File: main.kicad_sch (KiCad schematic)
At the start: 19 parts, among them SW1 Switch, SW2 Switch, SW3 Switch, SW4 Switch, SW5 Switch, SW6 Switch, SW7 Switch, SW8 Switch, SW9 Switch

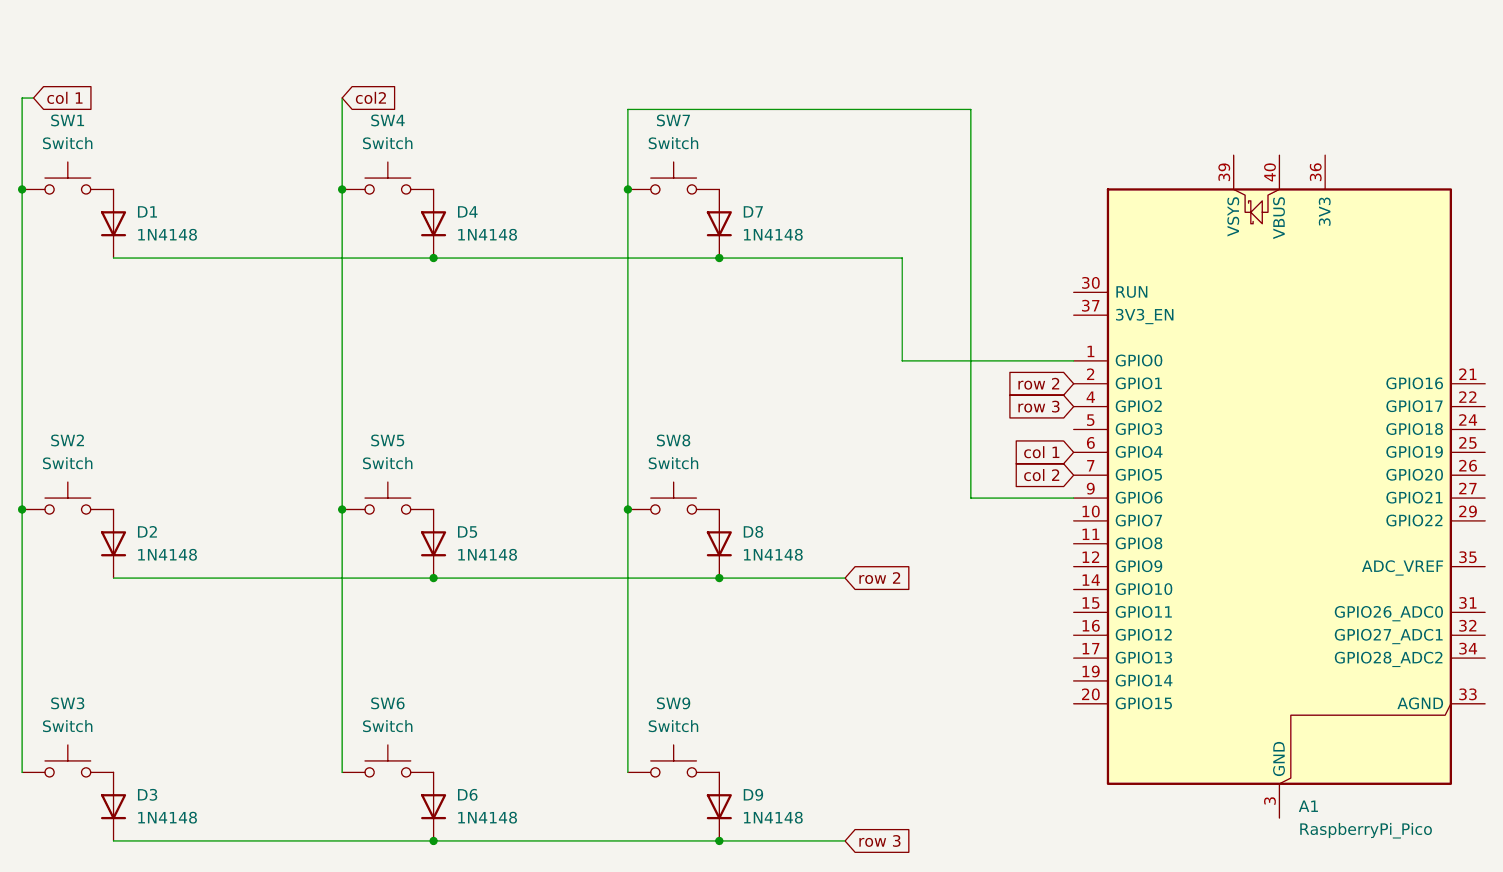
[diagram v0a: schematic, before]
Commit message: fixed pcb
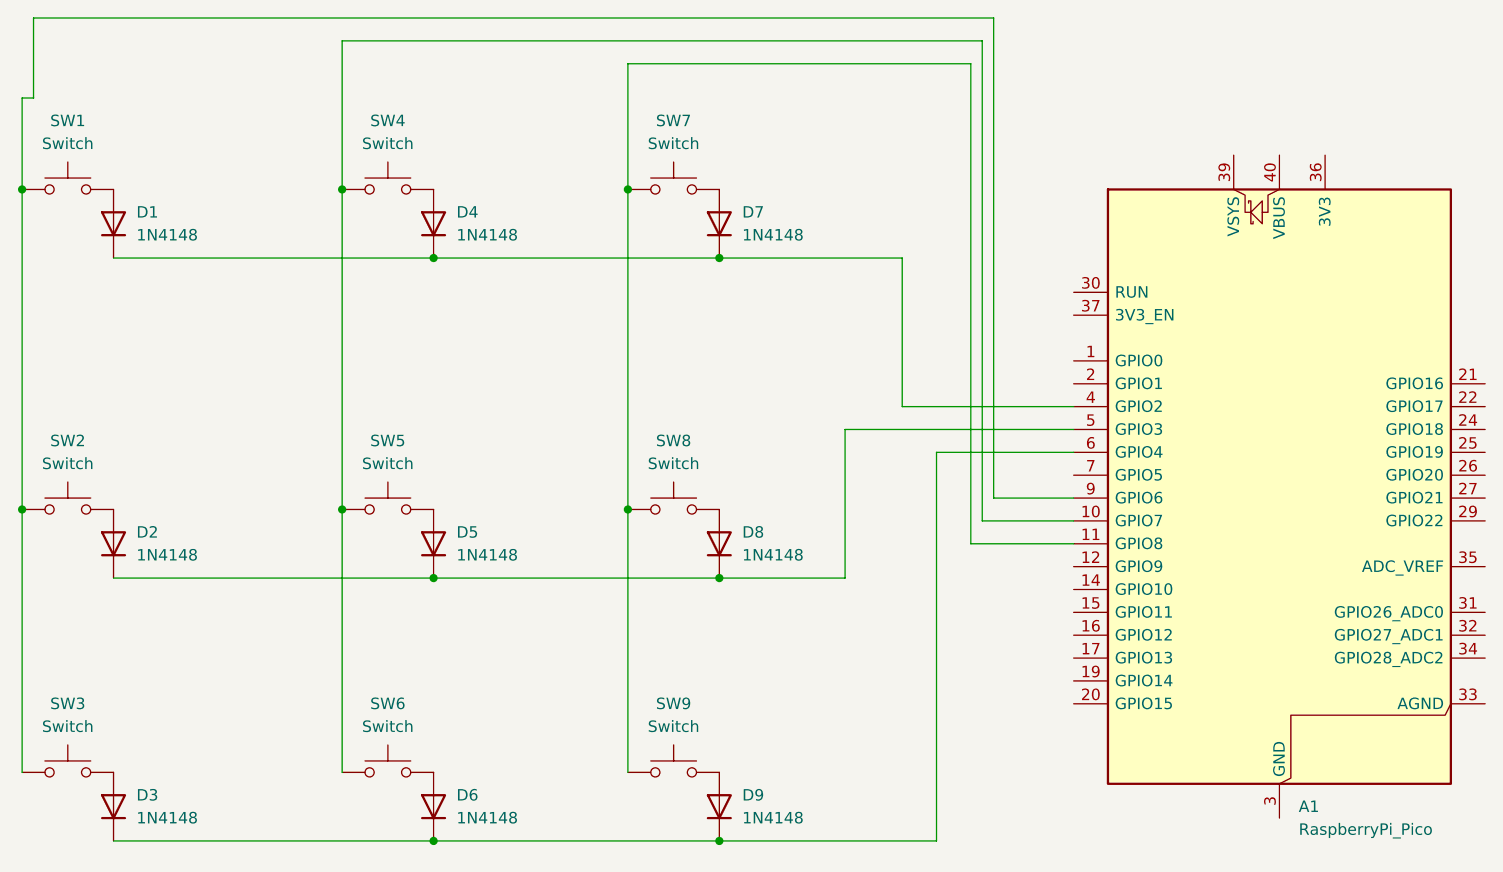
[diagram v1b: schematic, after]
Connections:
- net col2 is gone; now on an unnamed net: SW4.1, SW5.1, SW6.1
- net at D1.1 (K), D4.1 (K), D7.1 (K): now also A1.4 (GPIO2); no longer A1.1 (GPIO0)
- net at SW7.1, SW8.1, SW9.1: now also A1.11 (GPIO8); no longer A1.9 (GPIO6)
- net at A1.5 (GPIO3): now also D2.1 (K), D5.1 (K), D8.1 (K)
- net col 1: no longer names the net of SW1.1, SW2.1, SW3.1
- net col 1: now also A1.9 (GPIO6); no longer A1.6 (GPIO4)
- net col 2: no longer names the net of A1.7 (GPIO5)
- removed net row 2: A1.2 (GPIO1), D2.1 (K), D5.1 (K), D8.1 (K)
- net row 3: no longer names the net of D3.1 (K), D6.1 (K), D9.1 (K)
- net row 3: now also A1.6 (GPIO4); no longer A1.4 (GPIO2)
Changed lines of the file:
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@@
 	(wire
 		(pts
-			(xy 191.77 50.8) (xy 191.77 62.23)
+			(xy 95.25 24.13) (xy 201.93 24.13)
+		)
+		(stroke
+			(width 0)
+			(type default)
+		)
+	)
+	(wire
+		(pts
+			(xy 191.77 50.8) (xy 191.77 67.31)
+		)
+		(stroke
+			(width 0)
+			(type default)
+		)
+	)
+	(wire
+		(pts
+			(xy 195.58 115.57) (xy 195.58 72.39)
+		)
+		(stroke
+			(width 0)
+			(type default)
+		)
+	)
+	(wire
+		(pts
+			(xy 95.25 33.02) (xy 95.25 24.13)
 		)
 		(stroke
@@
 	(wire
 		(pts
-			(xy 199.39 34.29) (xy 161.29 34.29)
+			(xy 200.66 80.01) (xy 210.82 80.01)
+		)
+		(stroke
+			(width 0)
+			(type default)
+		)
+	)
+	(wire
+		(pts
+			(xy 199.39 29.21) (xy 199.39 82.55)
+		)
+		(stroke
+			(width 0)
+			(type default)
+		)
+	)
+	(wire
+		(pts
+			(xy 185.42 86.36) (xy 185.42 69.85)
+		)
+		(stroke
+			(width 0)
+			(type default)
+		)
+	)
+	(wire
+		(pts
+			(xy 200.66 26.67) (xy 200.66 80.01)
 		)
 		(stroke
@@
 	(wire
 		(pts
+			(xy 129.54 26.67) (xy 200.66 26.67)
+		)
+		(stroke
+			(width 0)
+			(type default)
+		)
+	)
+	(wire
+		(pts
 			(xy 95.25 33.02) (xy 93.98 33.02)
 		)
@@
 	(wire
 		(pts
-			(xy 199.39 34.29) (xy 199.39 77.47)
-		)
-		(stroke
-			(width 0)
-			(type default)
-		)
-	)
-	(wire
-		(pts
-			(xy 161.29 34.29) (xy 161.29 43.18)
-		)
-		(stroke
-			(width 0)
-			(type default)
-		)
-	)
-	(wire
-		(pts
 			(xy 93.98 33.02) (xy 93.98 43.18)
 		)
@@
 	(wire
 		(pts
-			(xy 199.39 77.47) (xy 210.82 77.47)
-		)
-		(stroke
-			(width 0)
-			(type default)
-		)
-	)
-	(wire
-		(pts
 			(xy 139.7 86.36) (xy 171.45 86.36)
 		)
@@
 	(wire
 		(pts
-			(xy 191.77 62.23) (xy 210.82 62.23)
+			(xy 195.58 72.39) (xy 210.82 72.39)
 		)
 		(stroke
@@
 	(wire
 		(pts
+			(xy 199.39 82.55) (xy 210.82 82.55)
+		)
+		(stroke
+			(width 0)
+			(type default)
+		)
+	)
+	(wire
+		(pts
+			(xy 185.42 69.85) (xy 210.82 69.85)
+		)
+		(stroke
+			(width 0)
+			(type default)
+		)
+	)
+	(wire
+		(pts
 			(xy 129.54 78.74) (xy 129.54 107.95)
 		)
@@
 	(wire
 		(pts
-			(xy 185.42 115.57) (xy 171.45 115.57)
+			(xy 201.93 24.13) (xy 201.93 77.47)
+		)
+		(stroke
+			(width 0)
+			(type default)
+		)
+	)
+	(wire
+		(pts
+			(xy 171.45 115.57) (xy 195.58 115.57)
+		)
+		(stroke
+			(width 0)
+			(type default)
+		)
+	)
+	(wire
+		(pts
+			(xy 161.29 29.21) (xy 161.29 43.18)
 		)
 		(stroke
@@
 	(wire
 		(pts
-			(xy 129.54 33.02) (xy 129.54 43.18)
+			(xy 201.93 77.47) (xy 210.82 77.47)
+		)
+		(stroke
+			(width 0)
+			(type default)
+		)
+	)
+	(wire
+		(pts
+			(xy 129.54 26.67) (xy 129.54 43.18)
 		)
 		(stroke
@@
 	(wire
 		(pts
+			(xy 161.29 29.21) (xy 199.39 29.21)
+		)
+		(stroke
+			(width 0)
+			(type default)
+		)
+	)
+	(wire
+		(pts
 			(xy 171.45 50.8) (xy 191.77 50.8)
 		)
@@
 		)
 	)
-	(global_label "row 3"
-		(shape input)
-		(at 210.82 67.31 180)
-		(fields_autoplaced yes)
-		(effects
-			(font
-				(size 1.27 1.27)
-			)
-			(justify right)
-		)
-		(property "Intersheetrefs" "${INTERSHEET_REFS}"
-			(at 202.392 67.31 0)
-			(effects
-				(font
-					(size 1.27 1.27)
-				)
-				(justify right)
-				(hide yes)
-			)
-		)
-	)
-	(global_label "row 3"
-		(shape input)
-		(at 185.42 115.57 0)
-		(fields_autoplaced yes)
-		(effects
-			(font
-				(size 1.27 1.27)
-			)
-			(justify left)
-		)
-		(property "Intersheetrefs" "${INTERSHEET_REFS}"
-			(at 193.848 115.57 0)
-			(effects
-				(font
-					(size 1.27 1.27)
-				)
-				(justify left)
-				(hide yes)
-			)
-		)
-	)
-	(global_label "col2"
-		(shape input)
-		(at 129.54 33.02 0)
-		(fields_autoplaced yes)
-		(effects
-			(font
-				(size 1.27 1.27)
-			)
-			(justify left)
-		)
-		(property "Intersheetrefs" "${INTERSHEET_REFS}"
-			(at 136.6375 33.02 0)
-			(effects
-				(font
-					(size 1.27 1.27)
-				)
-				(justify left)
-				(hide yes)
-			)
-		)
-	)
-	(global_label "row 2"
-		(shape input)
-		(at 210.82 64.77 180)
-		(fields_autoplaced yes)
-		(effects
-			(font
-				(size 1.27 1.27)
-			)
-			(justify right)
-		)
-		(property "Intersheetrefs" "${INTERSHEET_REFS}"
-			(at 202.392 64.77 0)
-			(effects
-				(font
-					(size 1.27 1.27)
-				)
-				(justify right)
-				(hide yes)
-			)
-		)
-	)
-	(global_label "col 1"
-		(shape input)
-		(at 95.25 33.02 0)
-		(fields_autoplaced yes)
-		(effects
-			(font
-				(size 1.27 1.27)
-			)
-			(justify left)
-		)
-		(property "Intersheetrefs" "${INTERSHEET_REFS}"
-			(at 103.3151 33.02 0)
-			(effects
-				(font
-					(size 1.27 1.27)
-				)
-				(justify left)
-				(hide yes)
-			)
-		)
-	)
-	(global_label "col 2"
-		(shape input)
-		(at 210.82 74.93 180)
-		(fields_autoplaced yes)
-		(effects
-			(font
-				(size 1.27 1.27)
-			)
-			(justify right)
-		)
-		(property "Intersheetrefs" "${INTERSHEET_REFS}"
-			(at 202.7549 74.93 0)
-			(effects
-				(font
-					(size 1.27 1.27)
-				)
-				(justify right)
-				(hide yes)
-			)
-		)
-	)
-	(global_label "col 1"
-		(shape input)
-		(at 210.82 72.39 180)
-		(fields_autoplaced yes)
-		(effects
-			(font
-				(size 1.27 1.27)
-			)
-			(justify right)
-		)
-		(property "Intersheetrefs" "${INTERSHEET_REFS}"
-			(at 202.7549 72.39 0)
-			(effects
-				(font
-					(size 1.27 1.27)
-				)
-				(justify right)
-				(hide yes)
-			)
-		)
-	)
-	(global_label "row 2"
-		(shape input)
-		(at 185.42 86.36 0)
-		(fields_autoplaced yes)
-		(effects
-			(font
-				(size 1.27 1.27)
-			)
-			(justify left)
-		)
-		(property "Intersheetrefs" "${INTERSHEET_REFS}"
-			(at 193.848 86.36 0)
-			(effects
-				(font
-					(size 1.27 1.27)
-				)
-				(justify left)
-				(hide yes)
-			)
-		)
-	)
+	(wire
+		(pts
+			(xy 191.77 67.31) (xy 210.82 67.31)
+		)
+		(stroke
+			(width 0)
+			(type default)
+		)
+	)
